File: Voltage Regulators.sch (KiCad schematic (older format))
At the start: 16 parts

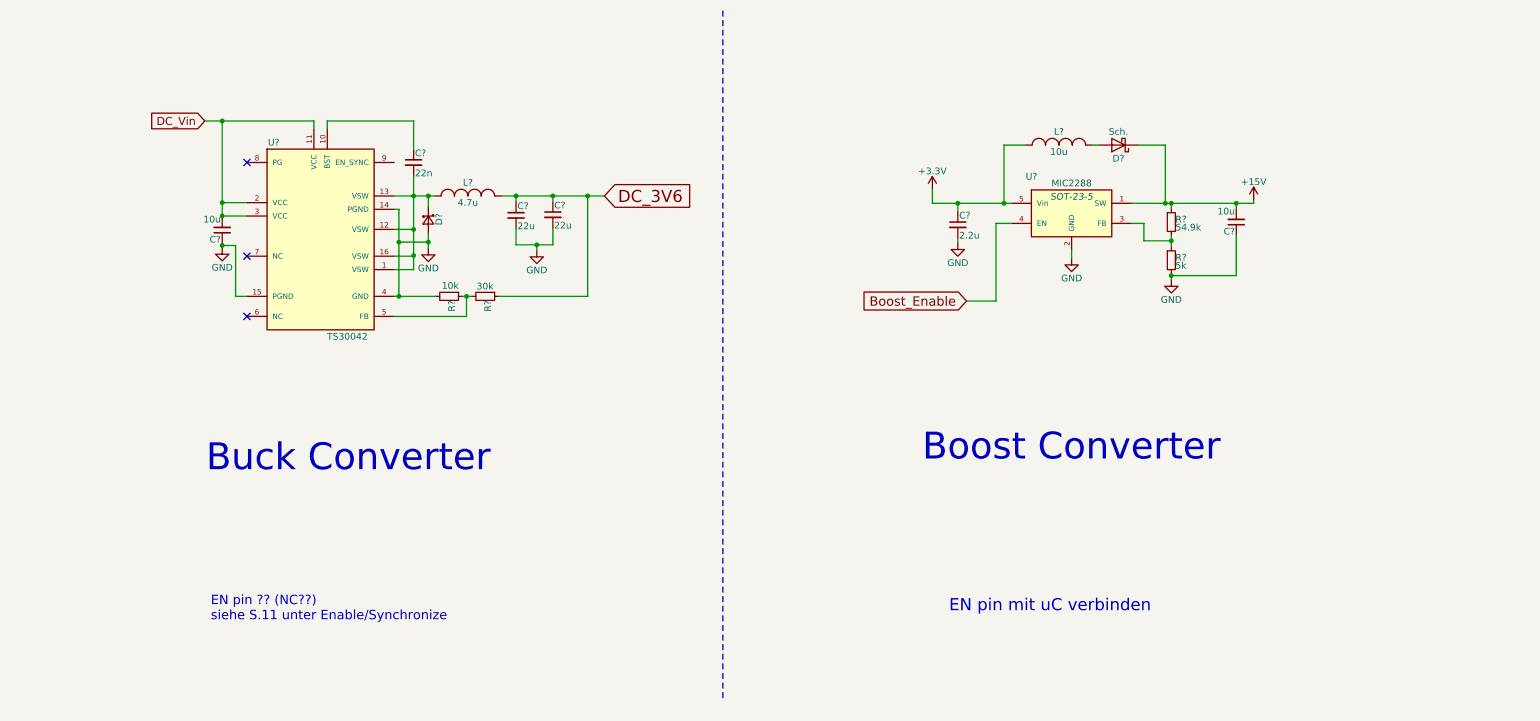
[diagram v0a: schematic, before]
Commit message: v1.0
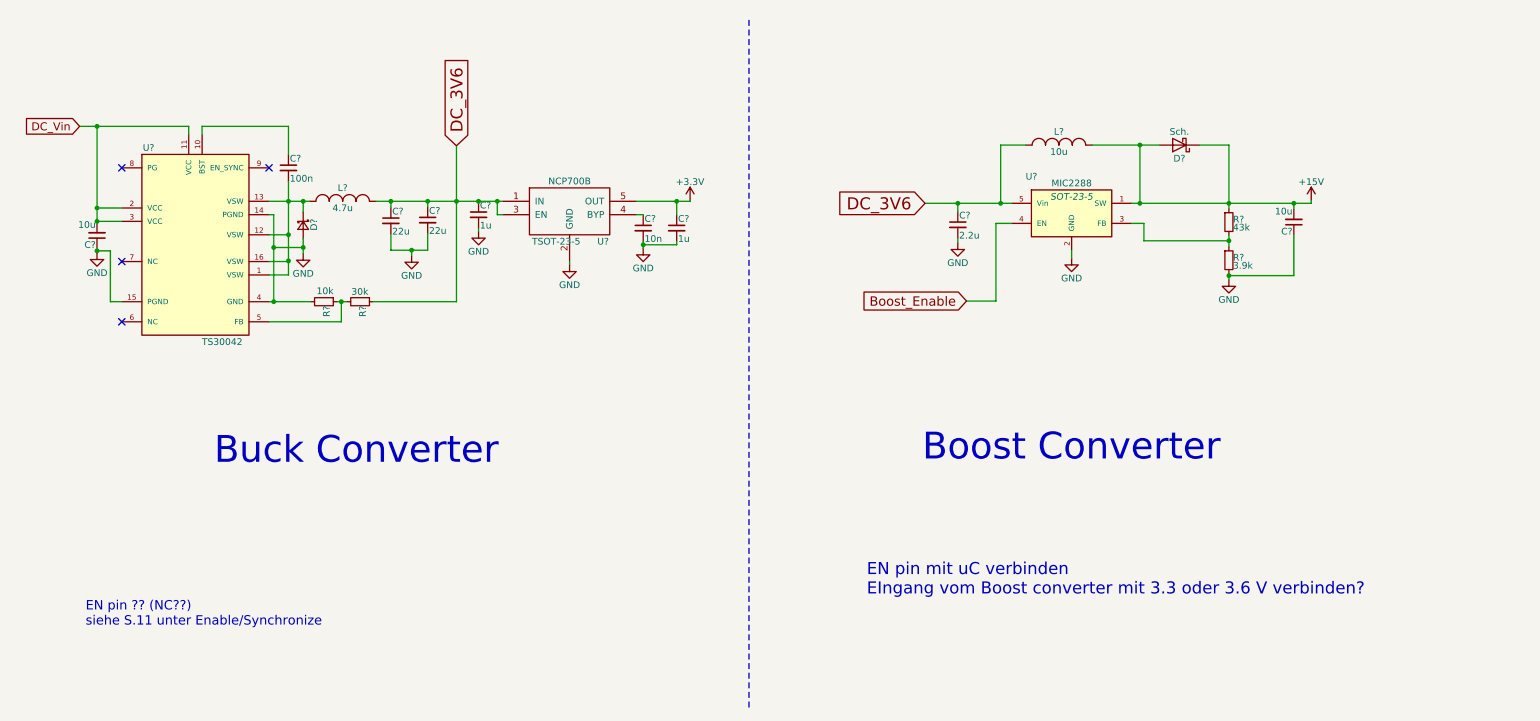
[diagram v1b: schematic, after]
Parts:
- added C?: 10n, symbol C_Small
- added C? (x2): 1u, symbol C_Small
- added U?: NCP700B, TSOT-23-5, symbol NCP700B
- C?: value 22n -> 100n
- R?: value 54.9k -> 43k
- R?: value 5k -> 3.9k
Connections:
- net +15V: now also D?.2 (A), L?.2
- net +3V3: now also C?.1, U?.5 (OUT); no longer C?.1, L?.1, U?.5 (Vin)
- net DC_3V6: now also C?.1, L?.1, U?.5 (Vin), C?.1, U?.1 (IN), U?.3 (EN)
- net GND: now also C?.2, C?.2, C?.2, U?.2 (GND)
- net at C?.2, D?.1 (K), L?.1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: no longer U?.16 (VSW)
- new net: C?.1, U?.4 (BYP)
- no-connect marks 3 -> 4
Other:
- note added: "EN pin mit uC verbinden\nEIngang vom Boost converter mit 3.3 oder 3.6 V verbinden?\n \n"
- note removed: "EN pin mit uC verbinden\n"
- moved on the sheet: C?, D?, L?, R?, U?
